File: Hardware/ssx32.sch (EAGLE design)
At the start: 86 parts, among them IC1 PIC18F45K20, IC2 FT232RL, IC3 TXB0108PW, IC4 TXB0108PW, IC5 TXB0108PW, IC6 TXB0108PW, IC7 78L33, IC8 74AHC1G08DBV, X1 8, X10 1, X11 19, X12 16, X13 15, X14 14, X15 13, X16 12, X17 11, X18 10, X19 9, X20 20, X21 21, X22 22, X23 23, X24 24, X25 25, X26 26, X27 27, X28 28, X29 29, X3 17, X30 30, X31 31, X32 32, X33 1751248, X34 18, X35 USB, X4 7, X5 6, X6 5, X7 4, X8 3, X9 2

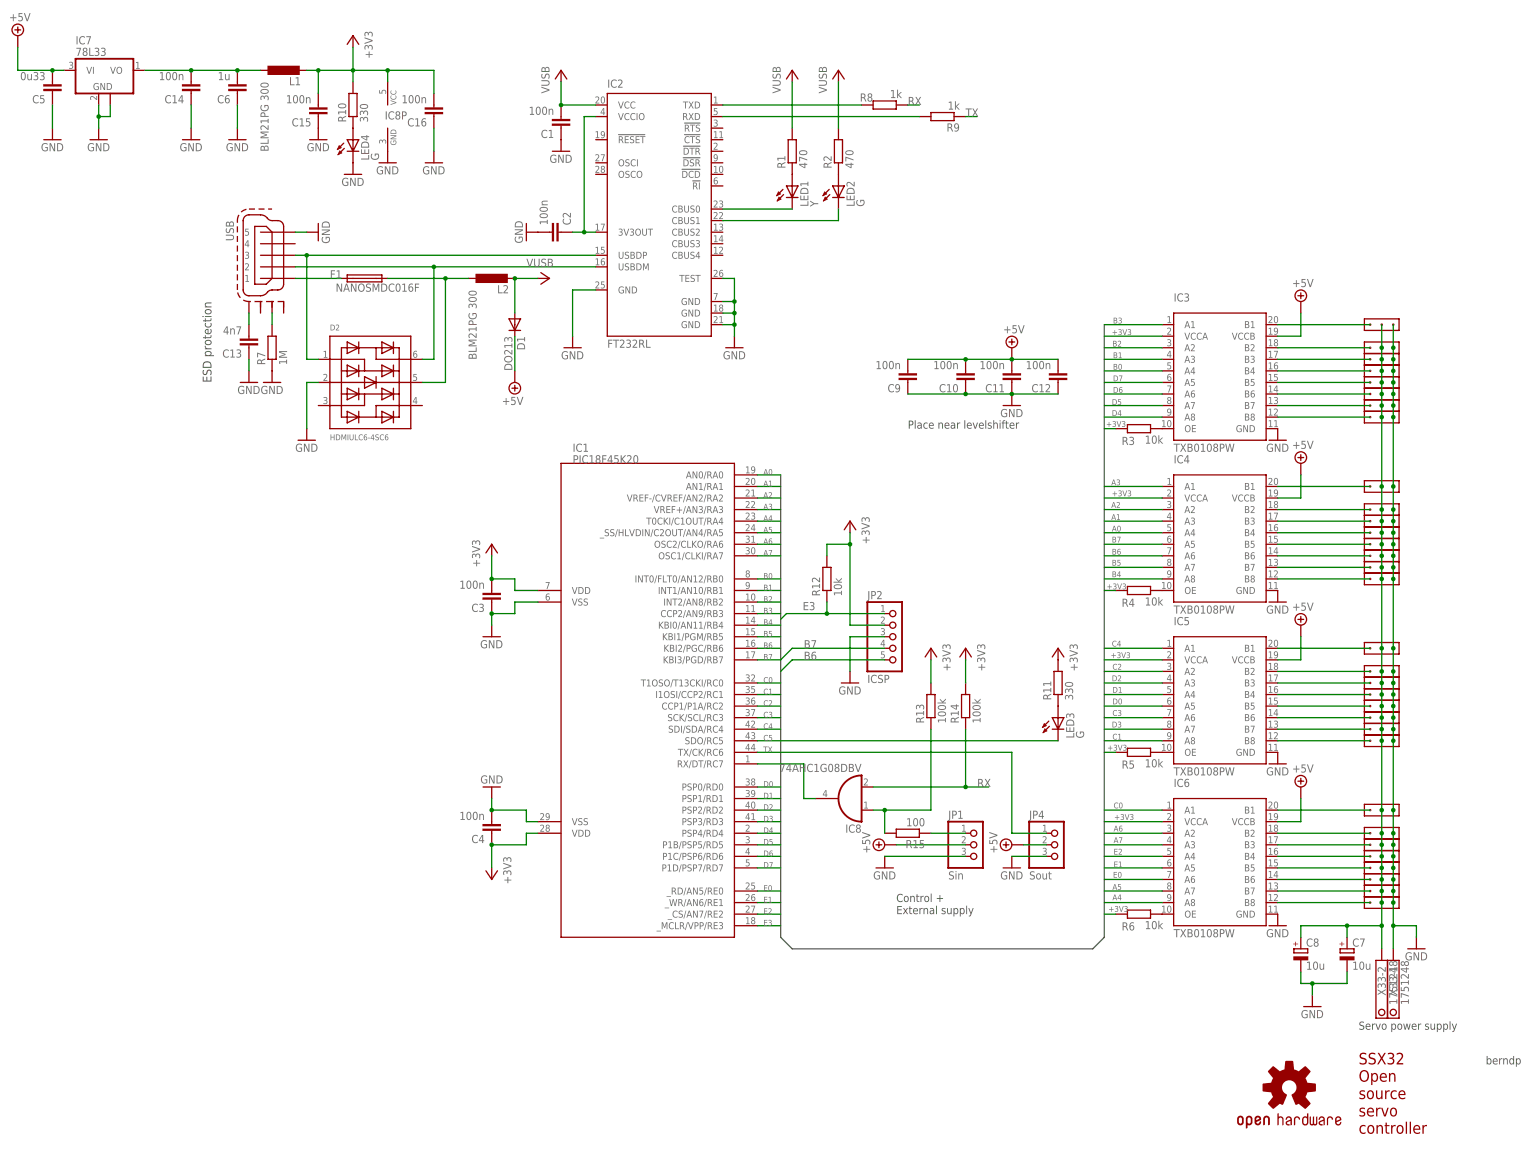
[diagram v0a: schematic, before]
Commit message: Revert "Fixed schematic errors"
This reverts commit bc55cbd2c08a143a3db725eeb6975bb6eadbf5e7.
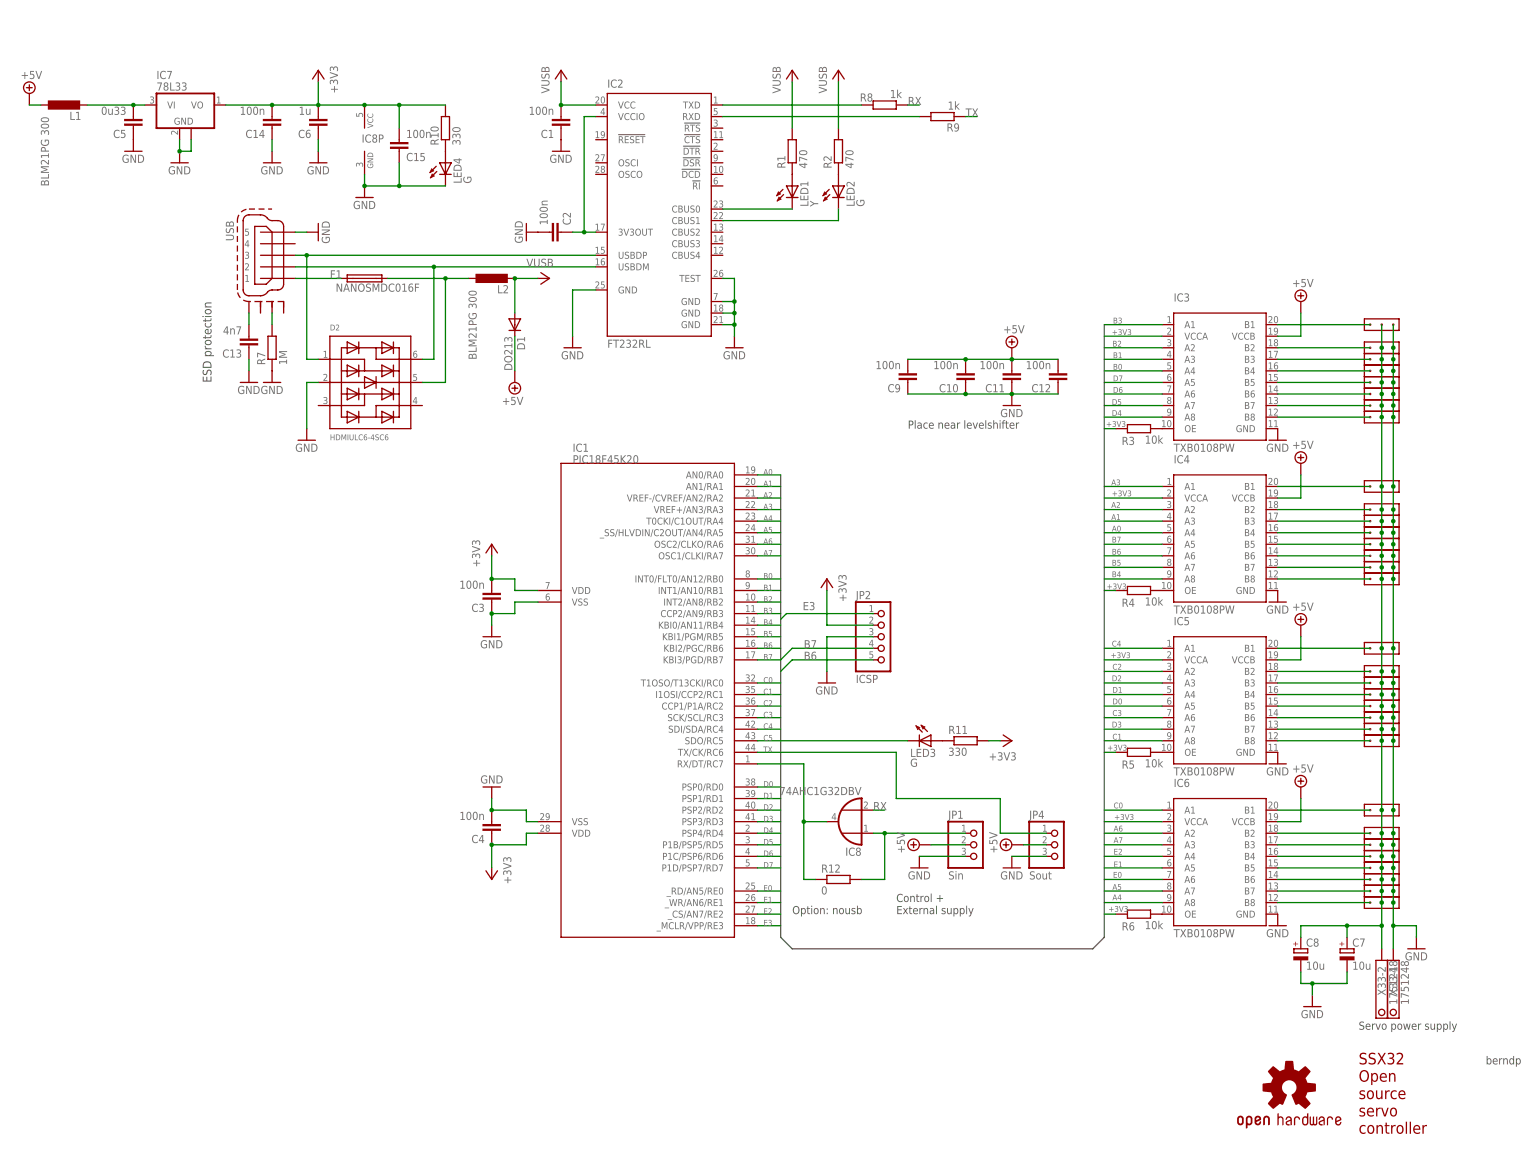
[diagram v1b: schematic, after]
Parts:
- removed C16: 100n, rcl:C-EUC0603
- removed R13, R14: 100k, rcl:R-EU_R0603
- removed R15: 100, rcl:R-EU_R0603
- IC8: value 74AHC1G08DBV -> 74AHC1G32DBV; device 74xx-little-de:74AHC1G08DBV -> 74xx-little-de:74AHC1G32DBV
- R12: value 10k -> 0
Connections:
- removed net N$42: IC1.RX/DT/RC7, IC8A.O
- removed net N$7: C14.2, C6.2, IC7.VO, L1.1
- new net N$54: IC8A.I0, JP1.1, R12.2
- net +3V3: now also C14.2, C6.2, IC7.VO; no longer C16.2, L1.2, R12.2, R13.2, R14.2
- net +UB: now also L1.1; no longer C5.2, IC7.VI
- net E3: no longer R12.1
- net GND: no longer C16.1
- net N$46: now also C5.2, IC7.VI, L1.2; no longer IC8A.I0, R13.1, R15.2
- net N$48: now also IC1.RX/DT/RC7, IC8A.O, R12.1; no longer JP1.1, R15.1
- net RX: no longer R14.1
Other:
- note added: "Option: nousb"
- moved on the sheet: C14, C15, C5, C6, IC7, IC8P, JP2, L1, LED3, LED4, R10, R11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

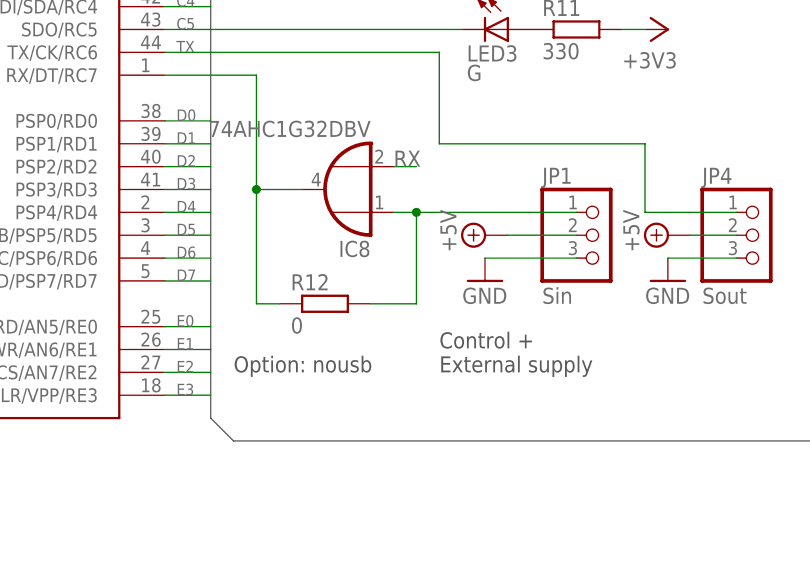
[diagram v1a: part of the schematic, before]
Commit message: Revert "Added software, minor board changes"
This reverts commit cd959f70c37cd81d74ff6deb02d888d0a529ccba.
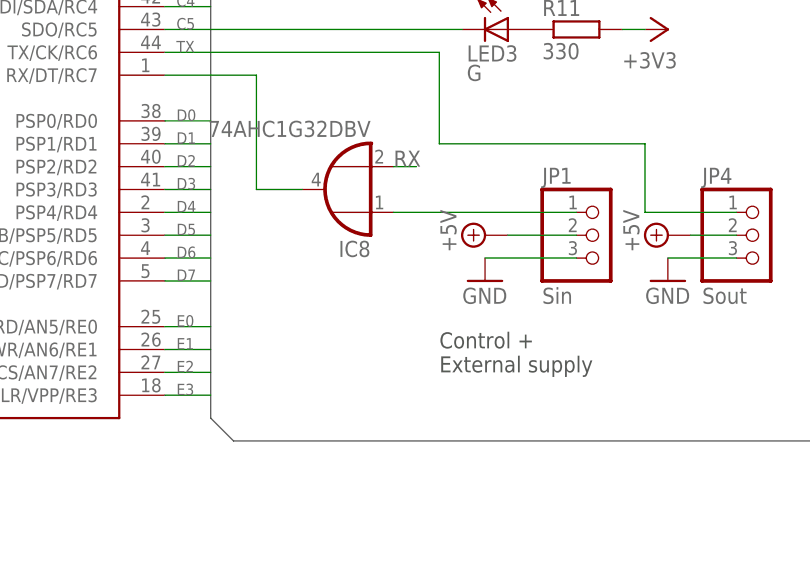
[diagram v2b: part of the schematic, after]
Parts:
- removed R12: 0, rcl:R-EU_R0603
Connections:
- net N$48: no longer R12.1
- net N$54: no longer R12.2
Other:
- note removed: "Option: nousb"
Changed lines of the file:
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@@
 <part name="LED4" library="led" deviceset="LED" device="CHIPLED_0603" value="G"/>
 <part name="R10" library="rcl" deviceset="R-EU_" device="R0603" value="330"/>
-<part name="R12" library="rcl" deviceset="R-EU_" device="R0603" value="0"/>
 </parts>
 <sheets>
@@
 <text x="172.72" y="50.8" size="1.778" layer="97">Control +
 External supply</text>
-<text x="149.86" y="50.8" size="1.778" layer="97">Option: nousb</text>
 </plain>
 <instances>
@@
 <instance part="LED4" gate="G$1" x="73.66" y="215.9"/>
 <instance part="R10" gate="G$1" x="73.66" y="223.52" rot="R90"/>
-<instance part="R12" gate="G$1" x="160.02" y="58.42"/>
 </instances>
 <busses>
@@
 <pinref part="JP1" gate="A" pin="1"/>
 <pinref part="IC8" gate="A" pin="I0"/>
-<wire x1="167.64" y1="68.58" x2="170.18" y2="68.58" width="0.1524" layer="91"/>
-<pinref part="R12" gate="G$1" pin="2"/>
-<wire x1="170.18" y1="68.58" x2="187.96" y2="68.58" width="0.1524" layer="91"/>
-<wire x1="165.1" y1="58.42" x2="170.18" y2="58.42" width="0.1524" layer="91"/>
-<wire x1="170.18" y1="58.42" x2="170.18" y2="68.58" width="0.1524" layer="91"/>
-<junction x="170.18" y="68.58"/>
+<wire x1="167.64" y1="68.58" x2="187.96" y2="68.58" width="0.1524" layer="91"/>
 </segment>
 </net>
@@
 <pinref part="IC1" gate="G$2" pin="RX/DT/RC7"/>
 <wire x1="152.4" y1="83.82" x2="142.24" y2="83.82" width="0.1524" layer="91"/>
-<pinref part="R12" gate="G$1" pin="1"/>
-<wire x1="154.94" y1="58.42" x2="152.4" y2="58.42" width="0.1524" layer="91"/>
-<wire x1="152.4" y1="58.42" x2="152.4" y2="71.12" width="0.1524" layer="91"/>
-<junction x="152.4" y="71.12"/>
-</segment>
-</net>
+</segment>
+</net>
